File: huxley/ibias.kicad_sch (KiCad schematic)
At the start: 24 parts, among them J21 61300211121, J25 61300211121, J26 61300211121, J27 61300211121, J28 61300211121, J29 61300211121, J30 61300211121, J31 61300211121, U2 LM134H, U4 TMUX1112PWR, U5 TMUX1112PWR

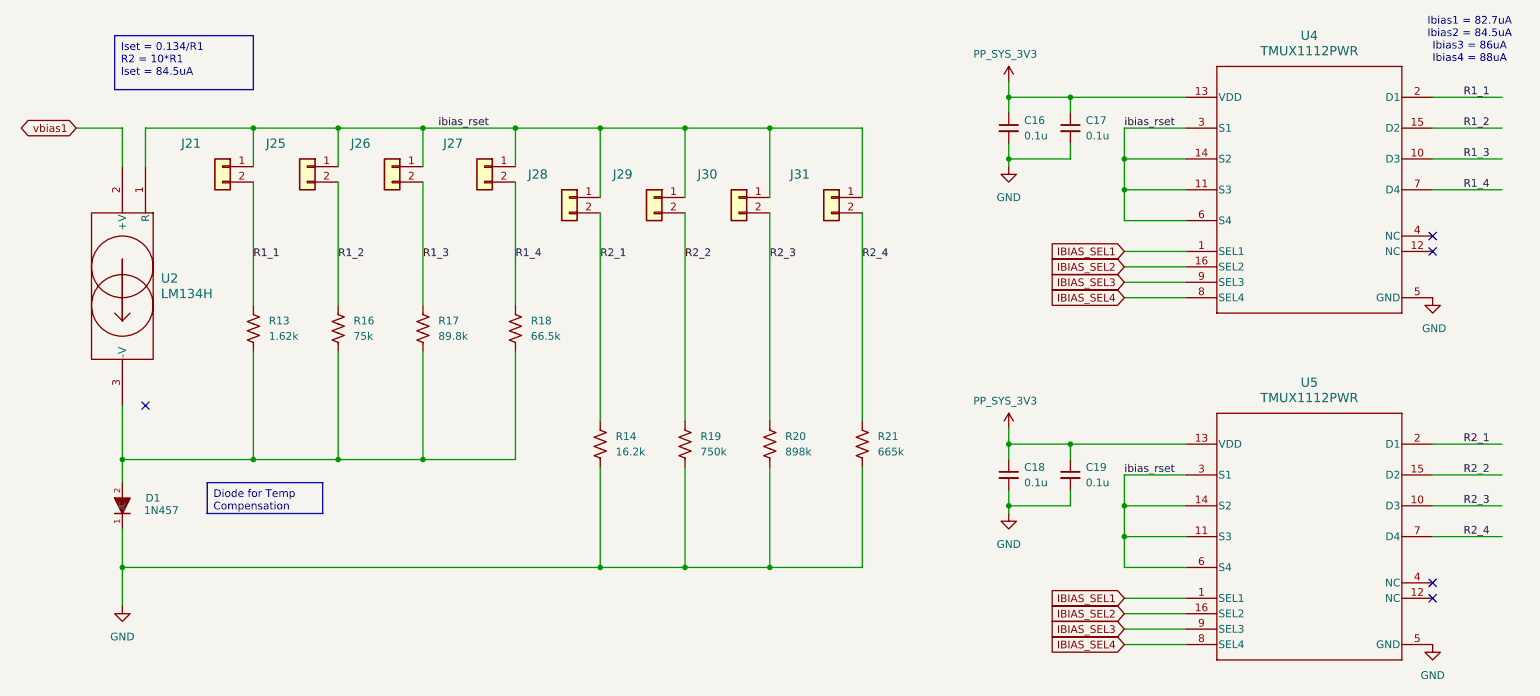
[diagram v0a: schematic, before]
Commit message: general rerrange struct inpl
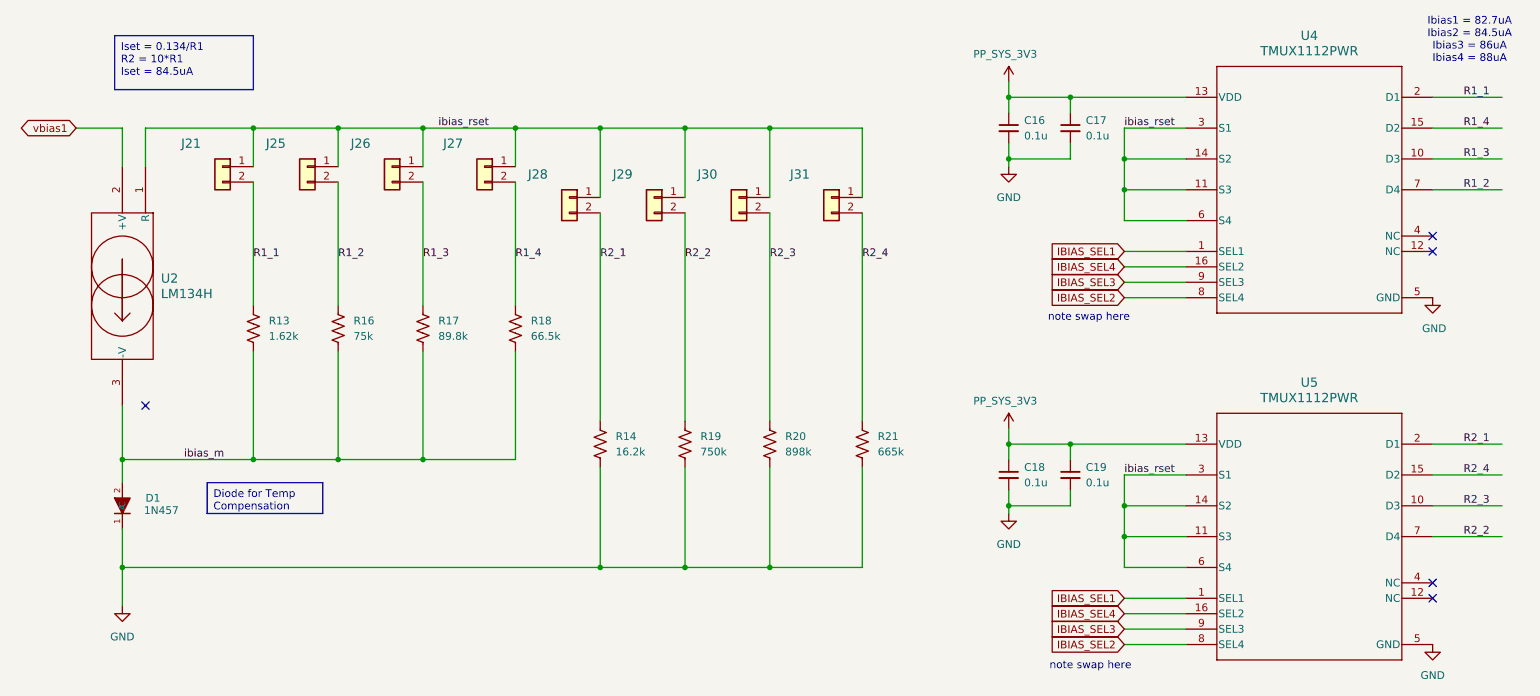
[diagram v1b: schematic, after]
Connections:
- net IBIAS_SEL2: now also U4.8 (SEL4), U5.8 (SEL4); no longer U4.16 (SEL2), U5.16 (SEL2)
- net IBIAS_SEL4: now also U4.16 (SEL2), U5.16 (SEL2); no longer U4.8 (SEL4), U5.8 (SEL4)
- net R1_2: now also U4.7 (D4); no longer U4.15 (D2)
- net R1_4: now also U4.15 (D2); no longer U4.7 (D4)
- net R2_2: now also U5.7 (D4); no longer U5.15 (D2)
- net R2_4: now also U5.15 (D2); no longer U5.7 (D4)
- net ibias_m: now reaches D1.2 (A), R13.2, R16.2, R17.2, R18.2, U2.3 (-V)
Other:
- note added: "note swap here"
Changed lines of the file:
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@@
+		)
+	)
+	(text "note swap here"
+		(exclude_from_sim no)
+		(at 194.818 80.772 0)
+		(effects
+			(font
+				(size 1.27 1.27)
+			)
+		)
+	)
+	(text "note swap here"
+		(exclude_from_sim no)
+		(at 195.072 138.176 0)
+		(effects
+			(font
+				(size 1.27 1.27)
+			)
 		)
 	)
@@
 		)
 	)
-	(label "R2_2"
+	(label "R2_4"
 		(at 256.54 106.68 0)
 		(fields_autoplaced yes)
@@
 		)
 	)
-	(label "R2_4"
+	(label "R2_2"
 		(at 256.54 116.84 0)
+		(fields_autoplaced yes)
+		(effects
+			(font
+				(size 1.27 1.27)
+			)
+			(justify left bottom)
+		)
+	)
+	(label "ibias_m"
+		(at 45.72 104.14 0)
 		(fields_autoplaced yes)
 		(effects
@@
 		)
 	)
+	(label "R1_2"
+		(at 256.54 59.69 0)
+		(fields_autoplaced yes)
+		(effects
+			(font
+				(size 1.27 1.27)
+			)
+			(justify left bottom)
+		)
+	)
 	(label "R1_4"
-		(at 256.54 59.69 0)
-		(fields_autoplaced yes)
-		(effects
-			(font
-				(size 1.27 1.27)
-			)
-			(justify left bottom)
-		)
-	)
-	(label "R1_2"
 		(at 256.54 49.53 0)
 		(fields_autoplaced yes)
@@
 		)
 	)
+	(global_label "IBIAS_SEL2"
+		(shape input)
+		(at 200.66 134.62 180)
+		(fields_autoplaced yes)
+		(effects
+			(font
+				(size 1.27 1.27)
+			)
+			(justify right)
+		)
+		(property "Intersheetrefs" "${INTERSHEET_REFS}"
+			(at 187.3334 134.62 0)
+			(effects
+				(font
+					(size 1.27 1.27)
+				)
+				(justify right)
+				(hide yes)
+			)
+		)
+	)
+	(global_label "IBIAS_SEL1"
+		(shape input)
+		(at 200.66 69.85 180)
+		(fields_autoplaced yes)
+		(effects
+			(font
+				(size 1.27 1.27)
+			)
+			(justify right)
+		)
+		(property "Intersheetrefs" "${INTERSHEET_REFS}"
+			(at 187.3334 69.85 0)
+			(effects
+				(font
+					(size 1.27 1.27)
+				)
+				(justify right)
+				(hide yes)
+			)
+		)
+	)
+	(global_label "IBIAS_SEL2"
+		(shape input)
+		(at 200.66 77.47 180)
+		(fields_autoplaced yes)
+		(effects
+			(font
+				(size 1.27 1.27)
+			)
+			(justify right)
+		)
+		(property "Intersheetrefs" "${INTERSHEET_REFS}"
+			(at 187.3334 77.47 0)
+			(effects
+				(font
+					(size 1.27 1.27)
+				)
+				(justify right)
+				(hide yes)
+			)
+		)
+	)
+	(global_label "IBIAS_SEL3"
+		(shape input)
+		(at 200.66 132.08 180)
+		(fields_autoplaced yes)
+		(effects
+			(font
+				(size 1.27 1.27)
+			)
+			(justify right)
+		)
+		(property "Intersheetrefs" "${INTERSHEET_REFS}"
+			(at 187.3334 132.08 0)
+			(effects
+				(font
+					(size 1.27 1.27)
+				)
+				(justify right)
+				(hide yes)
+			)
+		)
+	)
 	(global_label "IBIAS_SEL4"
-		(shape input)
-		(at 200.66 134.62 180)
-		(fields_autoplaced yes)
-		(effects
-			(font
-				(size 1.27 1.27)
-			)
-			(justify right)
-		)
-		(property "Intersheetrefs" "${INTERSHEET_REFS}"
-			(at 187.3334 134.62 0)
-			(effects
-				(font
-					(size 1.27 1.27)
-				)
-				(justify right)
-				(hide yes)
-			)
-		)
-	)
-	(global_label "IBIAS_SEL1"
-		(shape input)
-		(at 200.66 69.85 180)
-		(fields_autoplaced yes)
-		(effects
-			(font
-				(size 1.27 1.27)
-			)
-			(justify right)
-		)
-		(property "Intersheetrefs" "${INTERSHEET_REFS}"
-			(at 187.3334 69.85 0)
-			(effects
-				(font
-					(size 1.27 1.27)
-				)
-				(justify right)
-				(hide yes)
-			)
-		)
-	)
-	(global_label "IBIAS_SEL4"
-		(shape input)
-		(at 200.66 77.47 180)
-		(fields_autoplaced yes)
-		(effects
-			(font
-				(size 1.27 1.27)
-			)
-			(justify right)
-		)
-		(property "Intersheetrefs" "${INTERSHEET_REFS}"
-			(at 187.3334 77.47 0)
-			(effects
-				(font
-					(size 1.27 1.27)
-				)
-				(justify right)
-				(hide yes)
-			)
-		)
-	)
-	(global_label "IBIAS_SEL3"
-		(shape input)
-		(at 200.66 132.08 180)
-		(fields_autoplaced yes)
-		(effects
-			(font
-				(size 1.27 1.27)
-			)
-			(justify right)
-		)
-		(property "Intersheetrefs" "${INTERSHEET_REFS}"
-			(at 187.3334 132.08 0)
-			(effects
-				(font
-					(size 1.27 1.27)
-				)
-				(justify right)
-				(hide yes)
-			)
-		)
-	)
-	(global_label "IBIAS_SEL2"
 		(shape input)
 		(at 200.66 129.54 180)
@@
 		)
 	)
-	(global_label "IBIAS_SEL2"
+	(global_label "IBIAS_SEL4"
 		(shape input)
 		(at 200.66 72.39 180)
